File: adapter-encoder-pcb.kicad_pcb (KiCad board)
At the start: 4 copper layers, 14 x 15.6 mm, 33 parts, among them IC1 THVD2410VDRCR, M1 THRU_HOLE_PAD, M2 THRU_HOLE_PAD, U1 TLE5009E1000FUMA1, U2 STM32G031G6U6, U3 DF52-4S-0.8H(21), U4 SPX3819M5-L-3-3, U5 C2901617, U6 DF52-4S-0.8H(21), U7 SPX3819M5-L-3-3

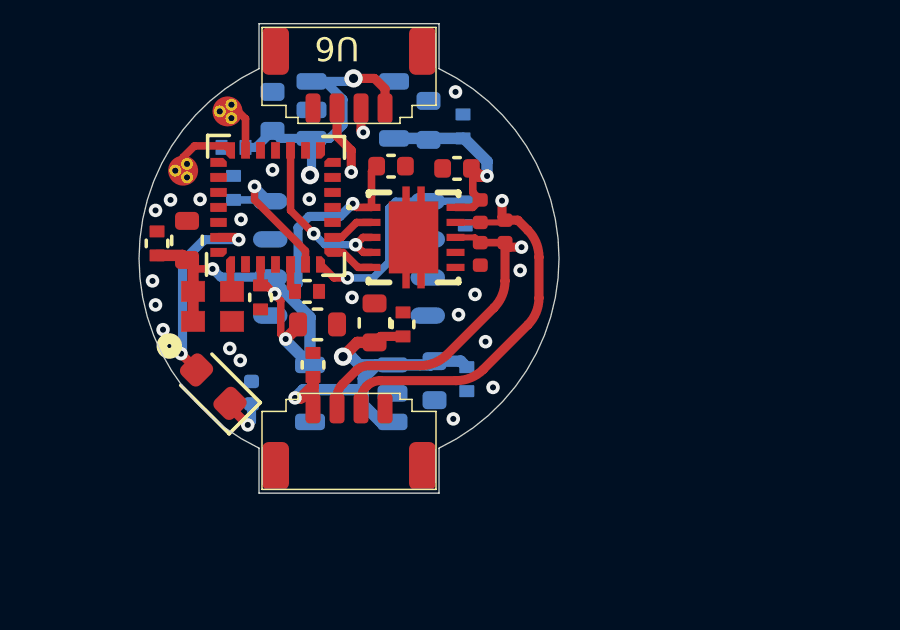
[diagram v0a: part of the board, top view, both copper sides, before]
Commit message: curves
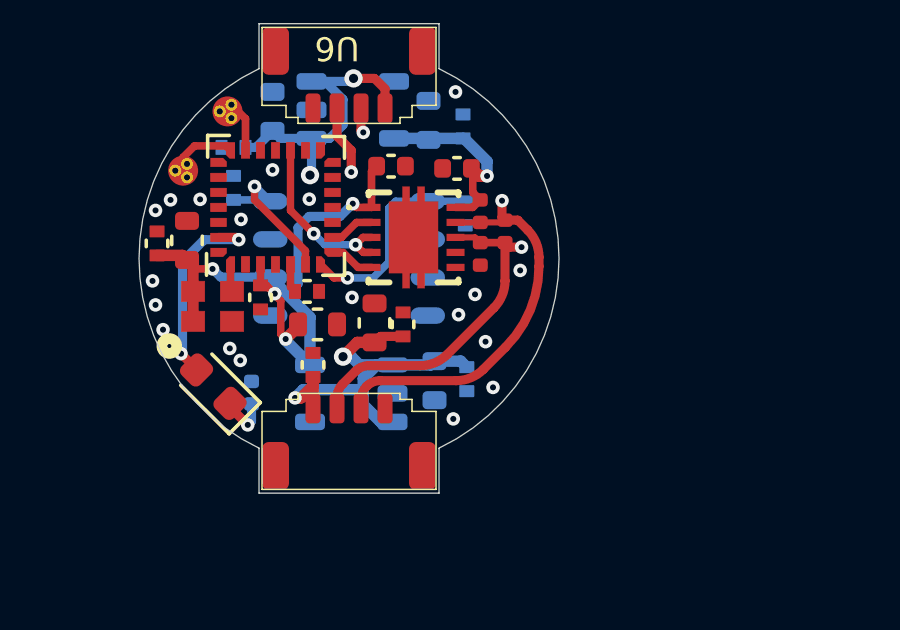
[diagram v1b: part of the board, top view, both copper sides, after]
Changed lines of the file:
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@@
   (segment (start 143.72885 110.81185) (end 144.098724 111.181724) (width 0.25) (layer "B.Cu") (net 22))
   (segment (start 143.727448 110.81185) (end 143.72885 110.81185) (width 0.25) (layer "B.Cu") (net 22))
-  (segment (start 145.304448 116.637448) (end 145.304448 116.350474) (width 0.3048) (layer "F.Cu") (net 23))
-  (segment (start 149.376423 115.340473) (end 150.864274 113.852622) (width 0.3048) (layer "F.Cu") (net 23))
+  (segment (start 150.529448 110.362448) (end 150.104448 110.362448) (width 0.3048) (layer "F.Cu") (net 23))
   (segment (start 144.504448 107.562448) (end 144.979108 108.037108) (width 0.3048) (layer "F.Cu") (net 23))
-  (segment (start 150.529448 110.362448) (end 150.104448 110.362448) (width 0.3048) (layer "F.Cu") (net 23))
   (segment (start 150.004448 110.262448) (end 150.104448 110.362448) (width 0.3048) (layer "F.Cu") (net 23))
+  (segment (start 145.490435 115.901461) (end 145.493461 115.898435) (width 0.3048) (layer "F.Cu") (net 23))
   (segment (start 145.942474 115.712448) (end 148.478397 115.712448) (width 0.3048) (layer "F.Cu") (net 23))
   (segment (start 144.979108 108.037108) (end 144.979108 108.760448) (width 0.3048) (layer "F.Cu") (net 23))
-  (segment (start 145.490435 115.901461) (end 145.493461 115.898435) (width 0.3048) (layer "F.Cu") (net 23))
   (segment (start 150.864273 110.697273) (end 150.529448 110.362448) (width 0.3048) (layer "F.Cu") (net 23))
   (segment (start 148.454448 110.437448) (end 149.279448 110.437448) (width 0.2032) (layer "F.Cu") (net 23))
   (segment (start 150.004448 109.712448) (end 150.004448 110.262448) (width 0.3048) (layer "F.Cu") (net 23))
+  (segment (start 149.376423 115.340473) (end 150.120325 114.596571) (width 0.3048) (layer "F.Cu") (net 23))
   (segment (start 144.504448 106.637448) (end 144.504448 107.562448) (width 0.3048) (layer "F.Cu") (net 23))
   (segment (start 149.279448 110.437448) (end 150.029448 110.437448) (width 0.2032) (layer "F.Cu") (net 23))
+  (segment (start 151.236248 111.902494) (end 151.236248 111.595299) (width 0.3048) (layer "F.Cu") (net 23))
+  (segment (start 145.304448 116.637448) (end 145.304448 116.350474) (width 0.3048) (layer "F.Cu") (net 23))
   (segment (start 150.029448 110.437448) (end 150.104448 110.362448) (width 0.2032) (layer "F.Cu") (net 23))
-  (segment (start 151.236248 112.954597) (end 151.236248 111.595299) (width 0.3048) (layer "F.Cu") (net 23))
   (via (at 144.979108 108.760448) (size 0.45) (drill 0.2) (layers "F.Cu" "B.Cu") (net 23))
   (via (at 150.004448 109.712448) (size 0.45) (drill 0.2) (layers "F.Cu" "B.Cu") (net 23))
-  (arc (start 145.490435 115.901461) (mid 145.352784 116.10747) (end 145.304448 116.350474) (width 0.3048) (layer "F.Cu") (net 23))
+  (arc (start 145.304448 116.350474) (mid 145.352784 116.10747) (end 145.490435 115.901461) (width 0.3048) (layer "F.Cu") (net 23))
+  (arc (start 145.493461 115.898435) (mid 145.69947 115.760784) (end 145.942474 115.712448) (width 0.3048) (layer "F.Cu") (net 23))
+  (arc (start 151.236248 111.902494) (mid 150.946229 113.360518) (end 150.120325 114.596571) (width 0.3048) (layer "F.Cu") (net 23))
   (arc (start 148.478397 115.712448) (mid 148.964405 115.615775) (end 149.376423 115.340473) (width 0.3048) (layer "F.Cu") (net 23))
-  (arc (start 150.864274 113.852622) (mid 151.139575 113.440605) (end 151.236248 112.954597) (width 0.3048) (layer "F.Cu") (net 23))
-  (arc (start 150.864273 110.697273) (mid 151.139575 111.109291) (end 151.236248 111.595299) (width 0.3048) (layer "F.Cu") (net 23))
-  (arc (start 145.493461 115.898435) (mid 145.69947 115.760784) (end 145.942474 115.712448) (width 0.3048) (layer "F.Cu") (net 23))
+  (arc (start 151.236248 111.595299) (mid 151.139575 111.109291) (end 150.864273 110.697273) (width 0.3048) (layer "F.Cu") (net 23))
   (segment (start 149.605499 109.712448) (end 150.004448 109.712448) (width 0.3048) (layer "In1.Cu") (net 23))
   (segment (start 144.979108 108.760448) (end 147.601397 108.760448) (width 0.3048) (layer "In1.Cu") (net 23))

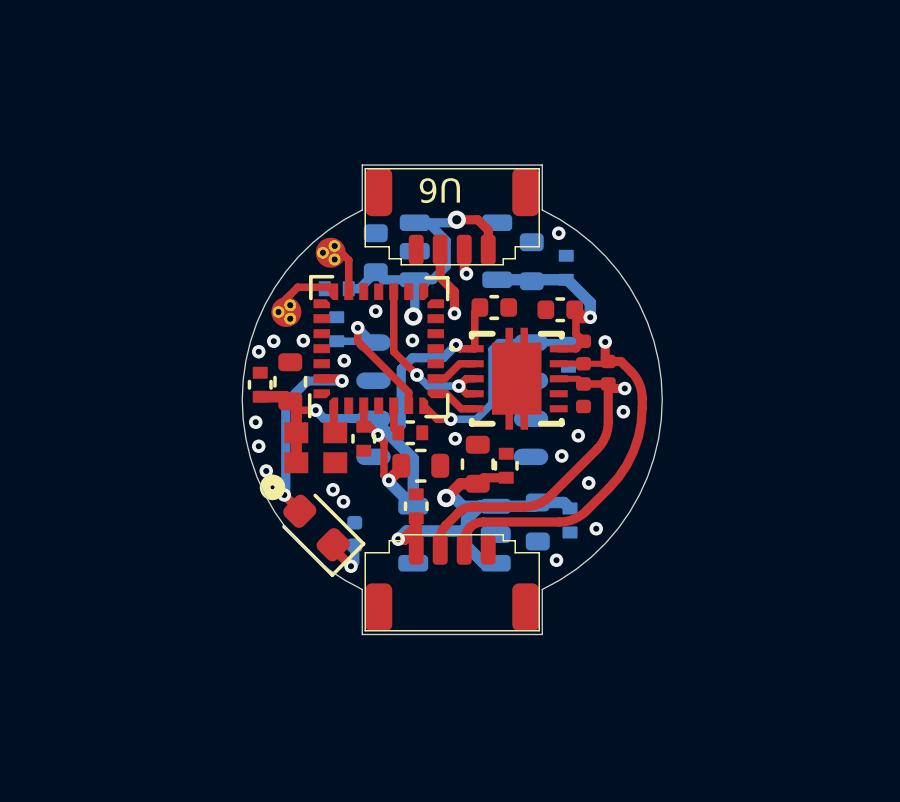
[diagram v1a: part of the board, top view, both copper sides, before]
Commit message: some minor tweaks
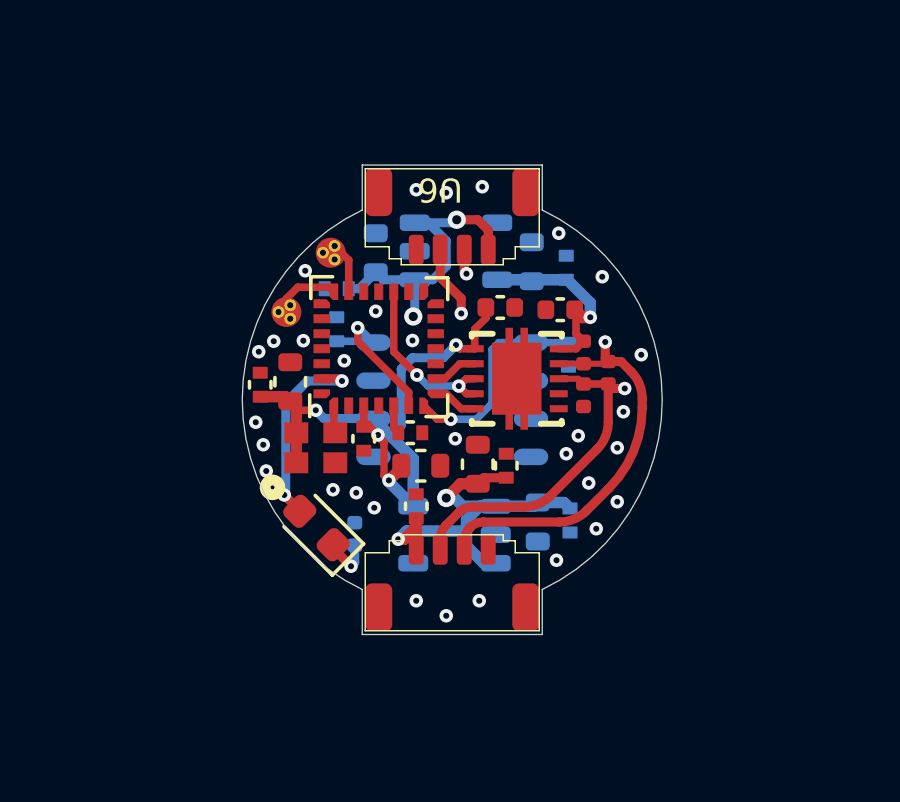
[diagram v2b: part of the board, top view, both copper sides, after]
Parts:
- moved C6 0.20 mm to (146.5, 108.6)
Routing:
- net GND: vias 19 -> 31
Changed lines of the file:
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@@
   )
   (footprint "Capacitor_SMD:C_0402_1005Metric" (layer "F.Cu")
-    (at 146.304448 108.562448 180)
+    (at 146.504448 108.562448 180)
     (descr "Capacitor SMD 0402 (1005 Metric), square (rectangular) end terminal, IPC_7351 nominal, (Body size source: IPC-SM-782 page 76, https://www.pcb-3d.com/wordpress/wp-content/uploads/ipc-sm-782a_amendment_1_and_2.pdf), generated with kicad-footprint-generator")
     (tags "capacitor")
@@
     (stroke (width 0.0254) (type solid)) (layer "Edge.Cuts"))
   (via (at 150.608848 112.037448) (size 0.45) (drill 0.2) (layers "F.Cu" "B.Cu") (net 1))
+  (via (at 144.704448 104.737448) (size 0.45) (drill 0.2) (layers "F.Cu" "B.Cu") (net 1))
   (via (at 148.379448 116.987448) (size 0.45) (drill 0.2) (layers "F.Cu" "B.Cu") (net 1))
-  (via (at 141.279448 115.037448) (size 0.45) (drill 0.2) (layers "F.Cu" "B.Cu") (net 1))
+  (via (at 141.704448 114.737448) (size 0.45) (drill 0.2) (layers "F.Cu" "B.Cu") (net 1))
   (via (at 140.929448 114.637448) (size 0.45) (drill 0.2) (layers "F.Cu" "B.Cu") (net 1))
   (via (at 141.304448 110.337448) (size 0.45) (drill 0.2) (layers "F.Cu" "B.Cu") (net 1))
   (via (at 138.954448 109.687448) (size 0.45) (drill 0.2) (layers "F.Cu" "B.Cu") (net 1))
   (via (at 149.704448 115.937448) (size 0.45) (drill 0.2) (layers "F.Cu" "B.Cu") (net 1))
+  (via (at 145.804448 118.337448) (size 0.45) (drill 0.2) (layers "F.Cu" "B.Cu") (net 1))
+  (via (at 140.004448 107.337448) (size 0.45) (drill 0.2) (layers "F.Cu" "B.Cu") (net 1))
+  (via (at 142.304448 115.237448) (size 0.45) (drill 0.2) (layers "F.Cu" "B.Cu") (net 1))
   (via (at 149.454448 114.412448) (size 0.45) (drill 0.2) (layers "F.Cu" "B.Cu") (net 1))
   (via (at 145.004448 112.937448) (size 0.45) (drill 0.2) (layers "F.Cu" "B.Cu") (net 1))
+  (via (at 143.704448 118.337448) (size 0.45) (drill 0.2) (layers "F.Cu" "B.Cu") (net 1))
   (via (at 138.704448 114.012448) (size 0.45) (drill 0.2) (layers "F.Cu" "B.Cu") (net 1))
   (via (at 149.104448 112.837448) (size 0.45) (drill 0.2) (layers "F.Cu" "B.Cu") (net 1))
-  (via (at 148.554448 113.512448) (size 0.45) (drill 0.2) (layers "F.Cu" "B.Cu") (net 1))
+  (via (at 144.704448 118.837448) (size 0.45) (drill 0.2) (layers "F.Cu" "B.Cu") (net 1))
+  (via (at 150.404448 115.037448) (size 0.45) (drill 0.2) (layers "F.Cu" "B.Cu") (net 1))
+  (via (at 148.704448 113.437448) (size 0.45) (drill 0.2) (layers "F.Cu" "B.Cu") (net 1))
   (via (at 139.940347 109.669538) (size 0.45) (drill 0.2) (layers "F.Cu" "B.Cu") (net 1))
+  (via (at 145.904448 104.537448) (size 0.45) (drill 0.2) (layers "F.Cu" "B.Cu") (net 1))
   (via (at 142.354448 108.687448) (size 0.45) (drill 0.2) (layers "F.Cu" "B.Cu") (net 1))
+  (via (at 143.704448 104.637448) (size 0.45) (drill 0.2) (layers "F.Cu" "B.Cu") (net 1))
   (via (at 138.354448 112.387448) (size 0.45) (drill 0.2) (layers "F.Cu" "B.Cu") (net 1))
   (via (at 148.454448 106.087448) (size 0.45) (drill 0.2) (layers "F.Cu" "B.Cu") (net 1))
   (via (at 138.454448 110.037448) (size 0.45) (drill 0.2) (layers "F.Cu" "B.Cu") (net 1))
-  (via (at 138.454448 113.187448) (size 0.45) (drill 0.2) (layers "F.Cu" "B.Cu") (net 1))
+  (via (at 149.904448 107.537448) (size 0.45) (drill 0.2) (layers "F.Cu" "B.Cu") (net 1))
+  (via (at 138.604448 113.137448) (size 0.45) (drill 0.2) (layers "F.Cu" "B.Cu") (net 1))
+  (via (at 150.404448 113.237448) (size 0.45) (drill 0.2) (layers "F.Cu" "B.Cu") (net 1))
+  (via (at 151.204448 110.137448) (size 0.45) (drill 0.2) (layers "F.Cu" "B.Cu") (net 1))
   (via (at 143.579448 109.662448) (size 0.45) (drill 0.2) (layers "F.Cu" "B.Cu") (net 1))
   (segment (start 144.854448 112.287448) (end 144.404448 112.287448) (width 0.25) (layer "F.Cu") (net 2))
@@
   (segment (start 145.154448 109.937448) (end 145.654448 109.937448) (width 0.254) (layer "F.Cu") (net 12))
   (segment (start 143.204448 113.912448) (end 143.204448 113.837448) (width 0.381) (layer "F.Cu") (net 12))
+  (segment (start 145.654448 109.287448) (end 146.024448 108.917448) (width 0.254) (layer "F.Cu") (net 12))
   (segment (start 145.029448 109.812448) (end 145.154448 109.937448) (width 0.254) (layer "F.Cu") (net 12))
   (segment (start 139.354448 111.537448) (end 139.504448 111.687448) (width 0.381) (layer "F.Cu") (net 12))
@@
   (segment (start 142.629448 114.162448) (end 142.629448 113.054878) (width 0.25) (layer "F.Cu") (net 12))
   (segment (start 142.791948 114.324948) (end 143.204448 113.912448) (width 0.381) (layer "F.Cu") (net 12))
-  (segment (start 145.654448 109.937448) (end 145.654448 108.732448) (width 0.254) (layer "F.Cu") (net 12))
+  (segment (start 145.654448 109.937448) (end 145.654448 109.287448) (width 0.254) (layer "F.Cu") (net 12))
   (segment (start 142.429448 112.854878) (end 142.429448 112.812448) (width 0.25) (layer "F.Cu") (net 12))
-  (segment (start 145.654448 108.732448) (end 145.824448 108.562448) (width 0.254) (layer "F.Cu") (net 12))
   (segment (start 138.504448 111.537448) (end 139.354448 111.537448) (width 0.381) (layer "F.Cu") (net 12))
+  (segment (start 146.024448 108.917448) (end 146.024448 108.562448) (width 0.254) (layer "F.Cu") (net 12))
   (segment (start 141.954448 112.537448) (end 141.954448 111.837448) (width 0.25) (layer "F.Cu") (net 12))
   (segment (start 142.629448 113.054878) (end 142.429448 112.854878) (width 0.25) (layer "F.Cu") (net 12))
@@
   (segment (start 143.727448 110.81185) (end 143.72885 110.81185) (width 0.25) (layer "B.Cu") (net 22))
   (segment (start 150.529448 110.362448) (end 150.104448 110.362448) (width 0.3048) (layer "F.Cu") (net 23))
-  (segment (start 144.504448 107.562448) (end 144.979108 108.037108) (width 0.3048) (layer "F.Cu") (net 23))
   (segment (start 150.004448 110.262448) (end 150.104448 110.362448) (width 0.3048) (layer "F.Cu") (net 23))
   (segment (start 145.490435 115.901461) (end 145.493461 115.898435) (width 0.3048) (layer "F.Cu") (net 23))
+  (segment (start 145.204448 108.762237) (end 145.204448 108.262448) (width 0.3048) (layer "F.Cu") (net 23))
   (segment (start 145.942474 115.712448) (end 148.478397 115.712448) (width 0.3048) (layer "F.Cu") (net 23))
-  (segment (start 144.979108 108.037108) (end 144.979108 108.760448) (width 0.3048) (layer "F.Cu") (net 23))
   (segment (start 150.864273 110.697273) (end 150.529448 110.362448) (width 0.3048) (layer "F.Cu") (net 23))
   (segment (start 148.454448 110.437448) (end 149.279448 110.437448) (width 0.2032) (layer "F.Cu") (net 23))
   (segment (start 150.004448 109.712448) (end 150.004448 110.262448) (width 0.3048) (layer "F.Cu") (net 23))
   (segment (start 149.376423 115.340473) (end 150.120325 114.596571) (width 0.3048) (layer "F.Cu") (net 23))
-  (segment (start 144.504448 106.637448) (end 144.504448 107.562448) (width 0.3048) (layer "F.Cu") (net 23))
+  (segment (start 145.204448 108.262448) (end 144.504448 107.562448) (width 0.3048) (layer "F.Cu") (net 23))
   (segment (start 149.279448 110.437448) (end 150.029448 110.437448) (width 0.2032) (layer "F.Cu") (net 23))
   (segment (start 151.236248 111.902494) (end 151.236248 111.595299) (width 0.3048) (layer "F.Cu") (net 23))
+  (segment (start 144.504448 107.562448) (end 144.504448 106.637448) (width 0.3048) (layer "F.Cu") (net 23))
   (segment (start 145.304448 116.637448) (end 145.304448 116.350474) (width 0.3048) (layer "F.Cu") (net 23))
   (segment (start 150.029448 110.437448) (end 150.104448 110.362448) (width 0.2032) (layer "F.Cu") (net 23))
-  (via (at 144.979108 108.760448) (size 0.45) (drill 0.2) (layers "F.Cu" "B.Cu") (net 23))
+  (via (at 145.204448 108.762237) (size 0.45) (drill 0.2) (layers "F.Cu" "B.Cu") (net 23))
   (via (at 150.004448 109.712448) (size 0.45) (drill 0.2) (layers "F.Cu" "B.Cu") (net 23))
   (arc (start 145.304448 116.350474) (mid 145.352784 116.10747) (end 145.490435 115.901461) (width 0.3048) (layer "F.Cu") (net 23))
@@
   (arc (start 148.478397 115.712448) (mid 148.964405 115.615775) (end 149.376423 115.340473) (width 0.3048) (layer "F.Cu") (net 23))
   (arc (start 151.236248 111.595299) (mid 151.139575 111.109291) (end 150.864273 110.697273) (width 0.3048) (layer "F.Cu") (net 23))
+  (segment (start 145.204628 108.762057) (end 147.701221 108.762057) (width 0.3048) (layer "In1.Cu") (net 23))
+  (segment (start 148.499423 109.132423) (end 148.707474 109.340474) (width 0.3048) (layer "In1.Cu") (net 23))
   (segment (start 149.605499 109.712448) (end 150.004448 109.712448) (width 0.3048) (layer "In1.Cu") (net 23))
-  (segment (start 144.979108 108.760448) (end 147.601397 108.760448) (width 0.3048) (layer "In1.Cu") (net 23))
-  (segment (start 148.499423 109.132423) (end 148.707474 109.340474) (width 0.3048) (layer "In1.Cu") (net 23))
-  (arc (start 148.499423 109.132423) (mid 148.087405 108.857121) (end 147.601397 108.760448) (width 0.3048) (layer "In1.Cu") (net 23))
+  (segment (start 145.204448 108.762237) (end 145.204628 108.762057) (width 0.3048) (layer "In1.Cu") (net 23))
+  (arc (start 147.701221 108.762057) (mid 148.133098 108.877098) (end 148.499423 109.132423) (width 0.3048) (layer "In1.Cu") (net 23))
   (arc (start 148.707474 109.340474) (mid 149.119491 109.615775) (end 149.605499 109.712448) (width 0.3048) (layer "In1.Cu") (net 23))
   (segment (start 148.454448 110.937448) (end 149.104448 110.937448) (width 0.2032) (layer "F.Cu") (net 24))
